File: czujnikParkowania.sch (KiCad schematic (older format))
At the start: 43 parts, among them J1 Screw_Terminal_01x03, Q1 BC817, Q2 IRF7404, Q3 BC817, Q4 BC817, Q5 BC817, SW1 SW_Push, U1 DC56-11SEKWA, U2 LM7805_TO220, U3 HC-SR04

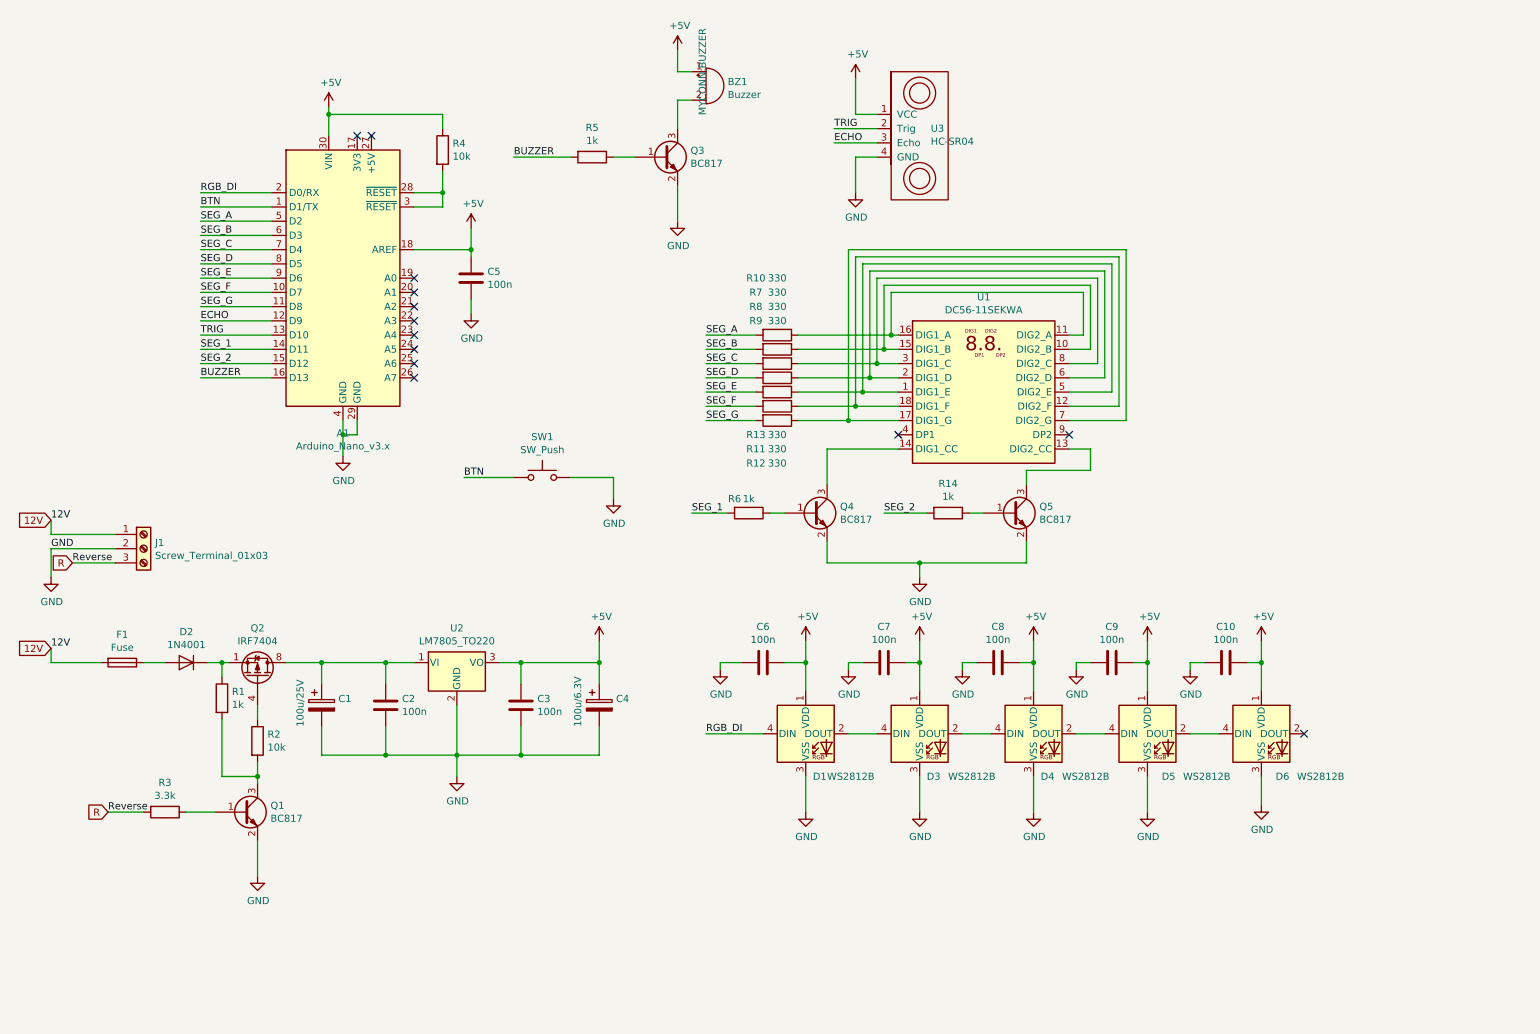
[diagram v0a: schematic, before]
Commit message: added GND plane on back
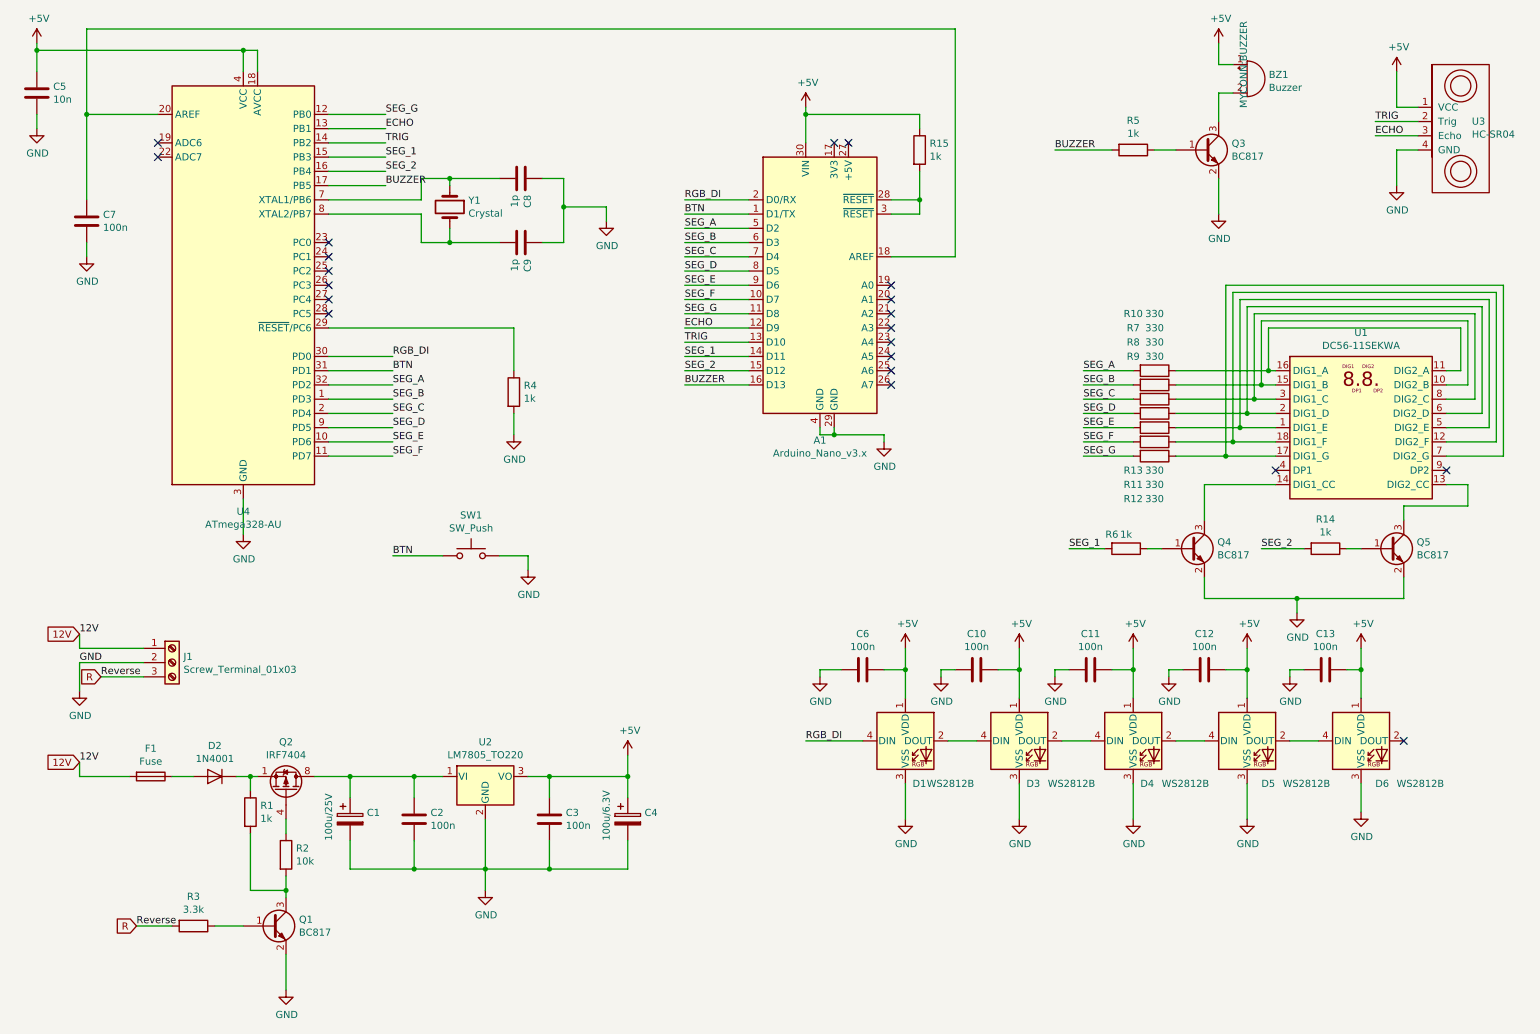
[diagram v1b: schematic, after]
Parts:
- added C11, C12, C13: 100n, Capacitor_SMD:C_0805_2012Metric, symbol Device:C
- added R15: 1k, Resistor_SMD:R_0805_2012Metric, symbol Device:R
- added U4: ATmega328-AU, Package_QFP:TQFP-32_7x7mm_P0.8mm, symbol MCU_Microchip_ATmega:ATmega328-AU
- added Y1: Crystal, MYCONN:16MHz cristal oscillator, symbol Device:Crystal
- C5: value 100n -> 10n
- C8, C9: value 100n -> 1p
- R4: value 10k -> 1k
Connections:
- net +5V: now also C11.1, C12.1, C13.1, R15.1, U4.18 (AVCC), U4.4 (VCC), U4.6 (VCC); no longer A1.18 (AREF), C7.1, C8.1, C9.1, R4.1
- net BTN: now also U4.31 (PD1)
- net BUZZER: now also U4.17 (PB5)
- net ECHO: now also U4.13 (PB1)
- net GND: now also C8.1, C9.1, R4.2, C11.2, C12.2, C13.2, U4.21 (GND), U4.3 (GND), U4.5 (GND); no longer C8.2, C9.2
- net RGB_DI: now also U4.30 (PD0)
- net SEG_1: now also U4.15 (PB3)
- net SEG_2: now also U4.16 (PB4)
- net SEG_A: now also U4.32 (PD2)
- net SEG_B: now also U4.1 (PD3)
- net SEG_C: now also U4.2 (PD4)
- net SEG_D: now also U4.9 (PD5)
- net SEG_E: now also U4.10 (PD6)
- net SEG_F: now also U4.11 (PD7)
- net SEG_G: now also U4.12 (PB0)
- net TRIG: now also U4.14 (PB2)
- net at A1.28 (~RESET), A1.3 (~RESET): now also R15.2; no longer R4.2
- new net: A1.18 (AREF), C7.1, U4.20 (AREF)
- new net: R4.1, U4.29 (~RESET~/PC6)
- new net: C8.2, U4.7 (XTAL1/PB6), Y1.1
- new net: C9.2, U4.8 (XTAL2/PB7), Y1.2
- no-connect marks 13 -> 21
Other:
- moved on the sheet: BZ1, C1, C2, C3, C4, C5, C6, D1, D2, D3, D4, D5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

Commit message: added GND plane on back. wrong brd in prev upload
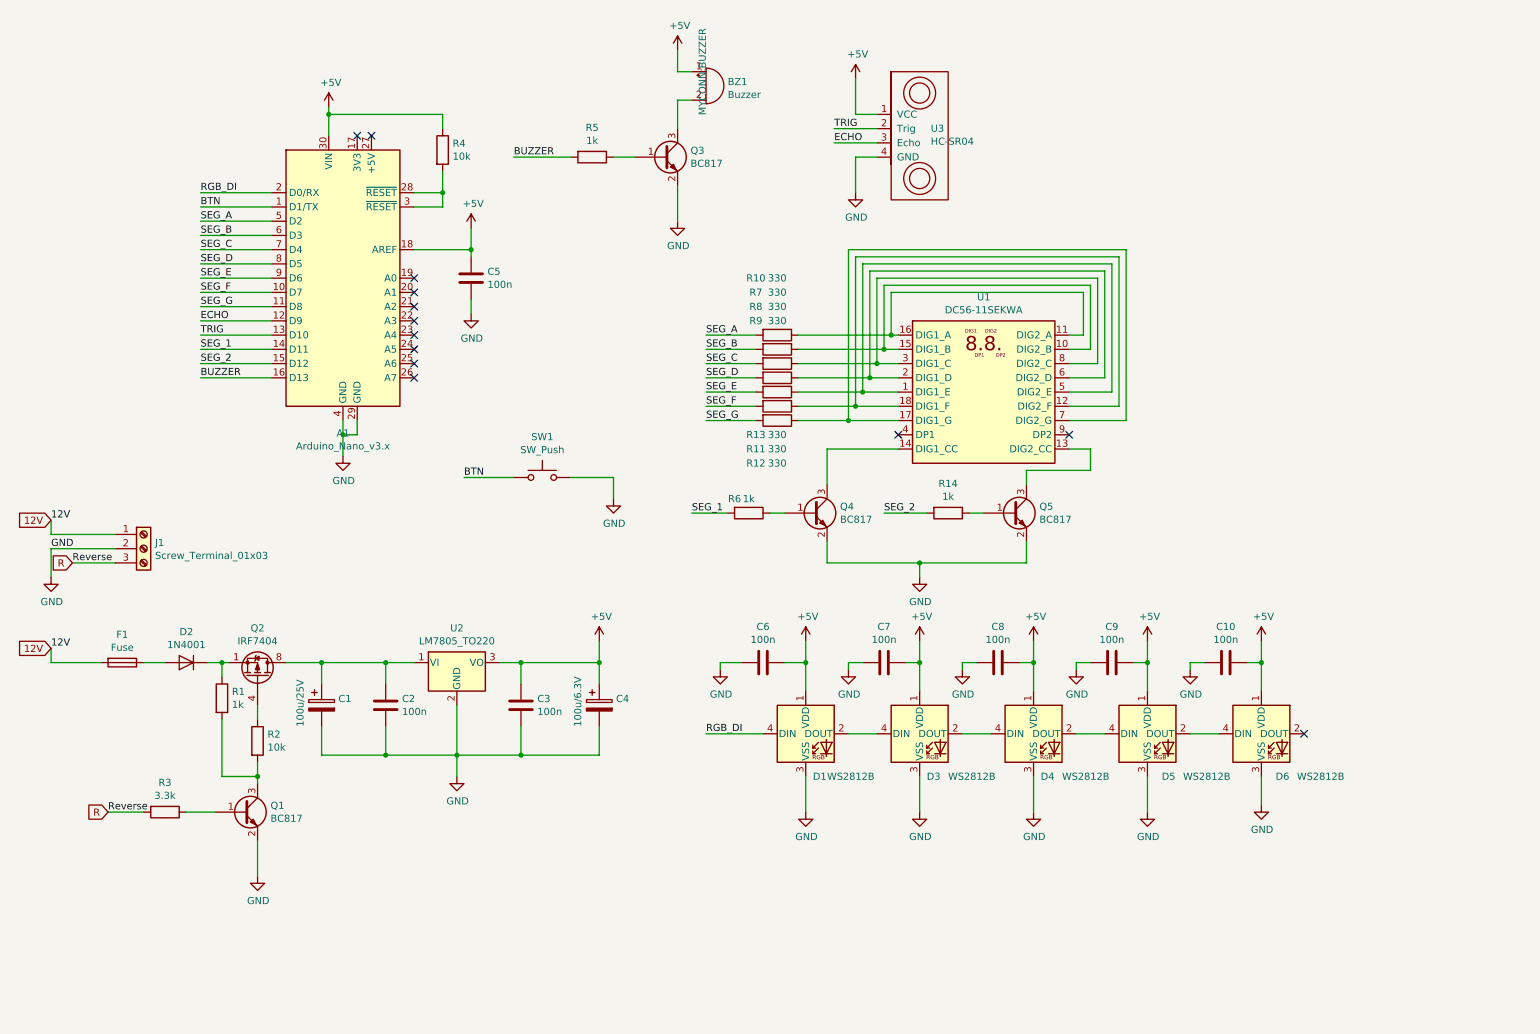
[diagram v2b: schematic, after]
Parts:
- removed C11, C12, C13: 100n, Capacitor_SMD:C_0805_2012Metric, symbol Device:C
- removed R15: 1k, Resistor_SMD:R_0805_2012Metric, symbol Device:R
- removed U4: ATmega328-AU, Package_QFP:TQFP-32_7x7mm_P0.8mm, symbol MCU_Microchip_ATmega:ATmega328-AU
- removed Y1: Crystal, MYCONN:16MHz cristal oscillator, symbol Device:Crystal
- C5: value 10n -> 100n
- C8, C9: value 1p -> 100n
- R4: value 1k -> 10k
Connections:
- net +5V: now also A1.18 (AREF), C7.1, C8.1, C9.1, R4.1
- net GND: now also C8.2, C9.2; no longer C8.1, C9.1, R4.2
- net at A1.28 (~RESET), A1.3 (~RESET): now also R4.2
- no-connect marks 21 -> 13
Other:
- moved on the sheet: BZ1, C1, C2, C3, C4, C5, C6, D1, D2, D3, D4, D5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
